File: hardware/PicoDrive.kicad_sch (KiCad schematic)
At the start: 55 parts, among them J1 M1, J2 M2, J3 M3, J4 RECEIVER, P1 USB_C_Plug_USB2.0, U1 W25Q32JVSS, U2 XC6206PxxxMR, U3 RP2040, U4 DRV8837, U5 DRV8837, U6 DRV8837, Y1 Crystal_GND2

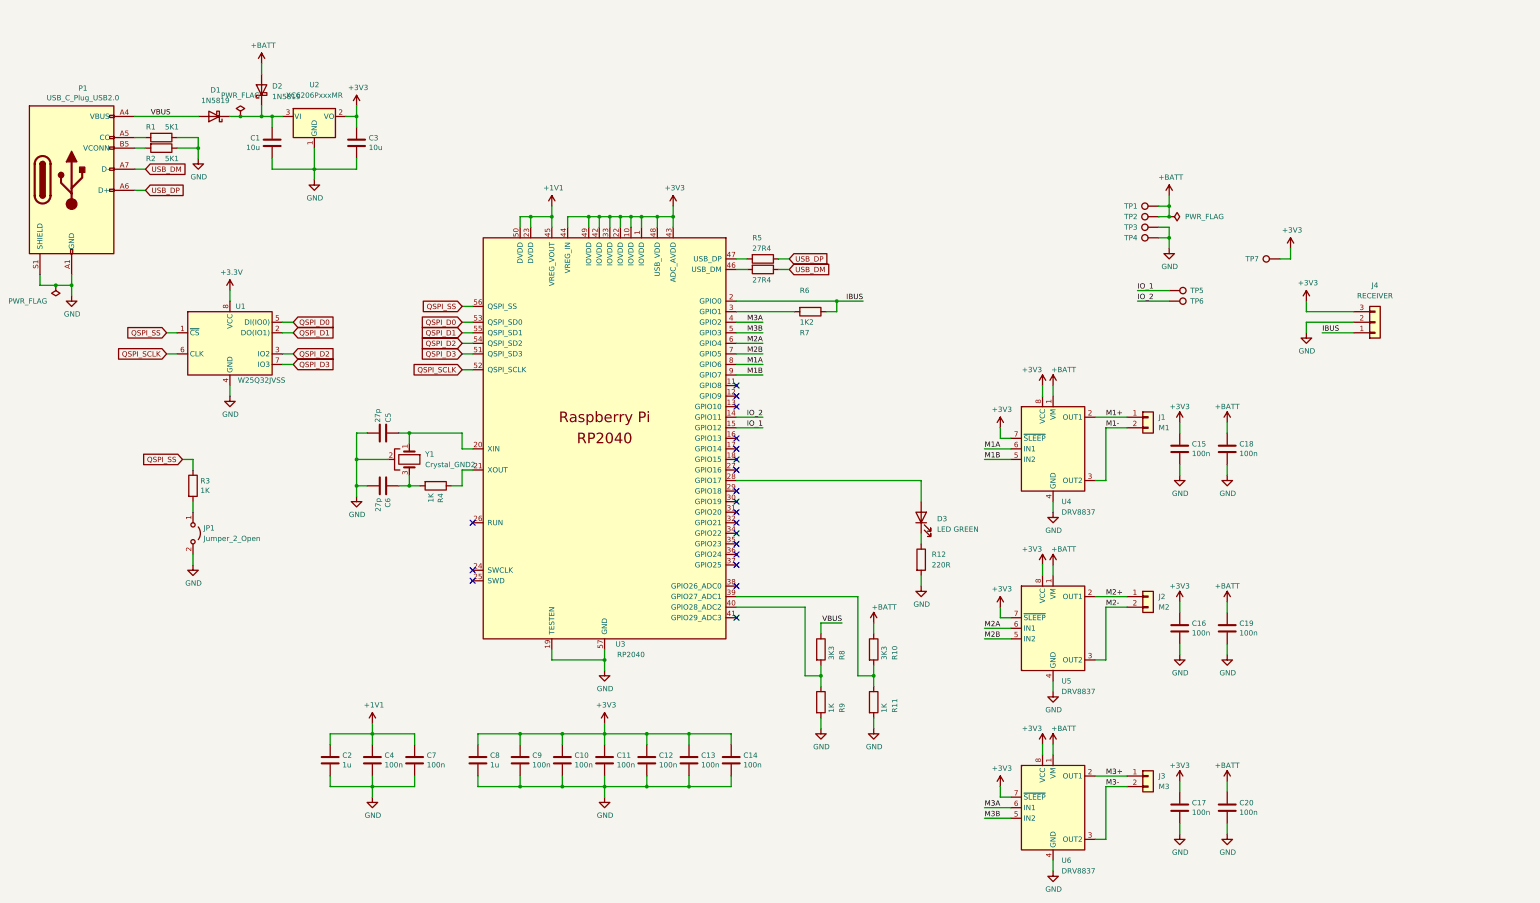
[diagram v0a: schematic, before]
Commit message: More firmware and some schematic updates
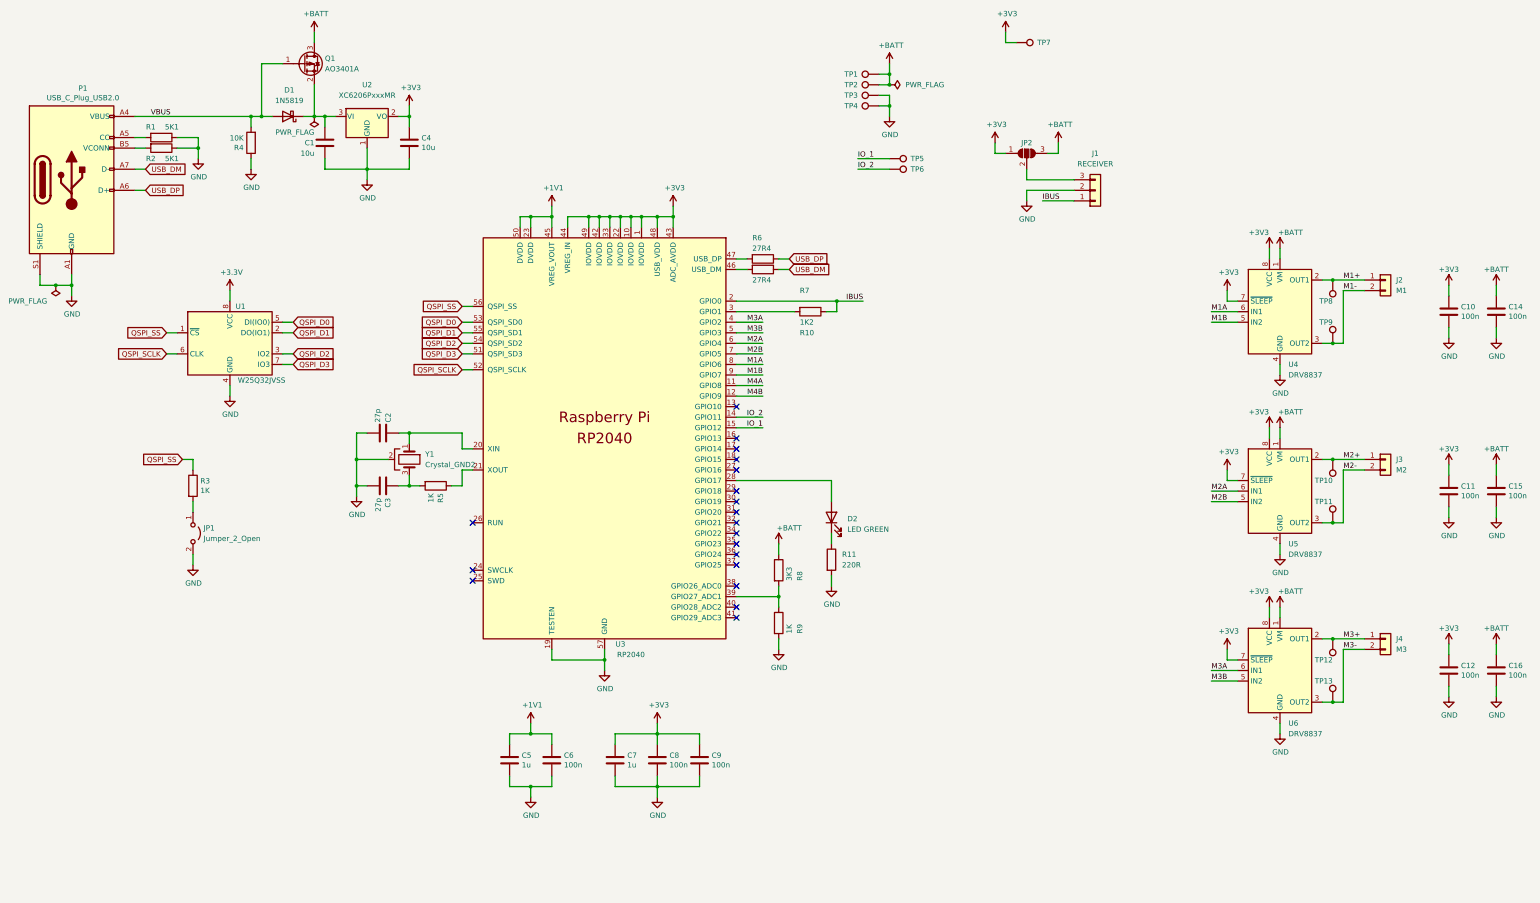
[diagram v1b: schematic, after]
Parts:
- removed C10, C13, C14, C9: 100n, Capacitor_SMD:C_0402_1005Metric, symbol Device:C
- removed C8: 1u, Capacitor_SMD:C_0402_1005Metric, symbol Device:C
- removed D2: 1N5819, Diode_SMD:D_SOD-323, symbol Diode:1N5819
- removed R8: 3K3, Resistor_SMD:R_0402_1005Metric, symbol Device:R
- removed R9: 1K, Resistor_SMD:R_0402_1005Metric, symbol Device:R
- added JP2: SolderJumper_3_Open, Jumper:SolderJumper-3_P1.3mm_Open_RoundedPad1.0x1.5mm, symbol Jumper:SolderJumper_3_Open
- added Q1: AO3401A, Package_TO_SOT_SMD:SOT-23, symbol Transistor_FET:AO3401A
- added R4: 10K, Resistor_SMD:R_0402_1005Metric, symbol Device:R
- added TP10, TP11, TP12, TP13, TP8, TP9: PWM2, TestPoint:TestPoint_Pad_1.5x1.5mm, symbol Connector:TestPoint
- C7: value 100n -> 1u
- renumbered C15 to C10, C16 to C11, C17 to C12, C18 to C14, C19 to C15, C20 to C16, C5 to C2, C6 to C3, C3 to C4, C2 to C5, C4 to C6, C11 to C8, C12 to C9, D3 to D2, J4 to J1, J1 to J2, J2 to J3, J3 to J4, R7 to R10, R12 to R11, R4 to R5, R5 to R6, R6 to R7, R10 to R8, R11 to R9
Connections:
- net +1V1: no longer C7.1
- net +3V3: now also C7.1, JP2.1 (A); no longer J1.3 (Pin_3)
- net +BATT: now also JP2.3 (B), Q1.3 (D)
- net GND: now also R4.1
- net M1+: now also TP8.1
- net M1-: now also TP9.1
- net M2+: now also TP10.1
- net M2-: now also TP11.1
- net M3+: now also TP12.1
- net M3-: now also TP13.1
- net VBUS: now also Q1.1 (G), R4.2
- net M4A: now reaches U3.11 (GPIO8)
- net M4B: now reaches U3.12 (GPIO9)
- net at C1.1, D1.1 (K), U2.3 (VI): now also Q1.2 (S)
- new net: J1.3 (Pin_3), JP2.2 (C)
- no-connect marks 20 -> 19
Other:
- moved on the sheet: C1, C10, C11, C12, C14, C15, C16, C4, C5, C6, C8, C9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
